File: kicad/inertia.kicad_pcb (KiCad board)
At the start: 2 copper layers, 87.9 x 91.7 mm, 35 parts, among them J10 Conn_01x02, J2 USB_C_Receptacle_USB2.0_16P, J3 Conn_01x02, J4 Conn_01x03, J5 Conn_01x02, J6 Conn_01x03, J7 Conn_01x02, J8 Conn_01x03, J9 Conn_01x02, SW1 SW_Push, SW2 SW_Push, U1 TJA1042T-3, U2 ESP32-S3-WROOM-1, U3 LSM6DSOTR

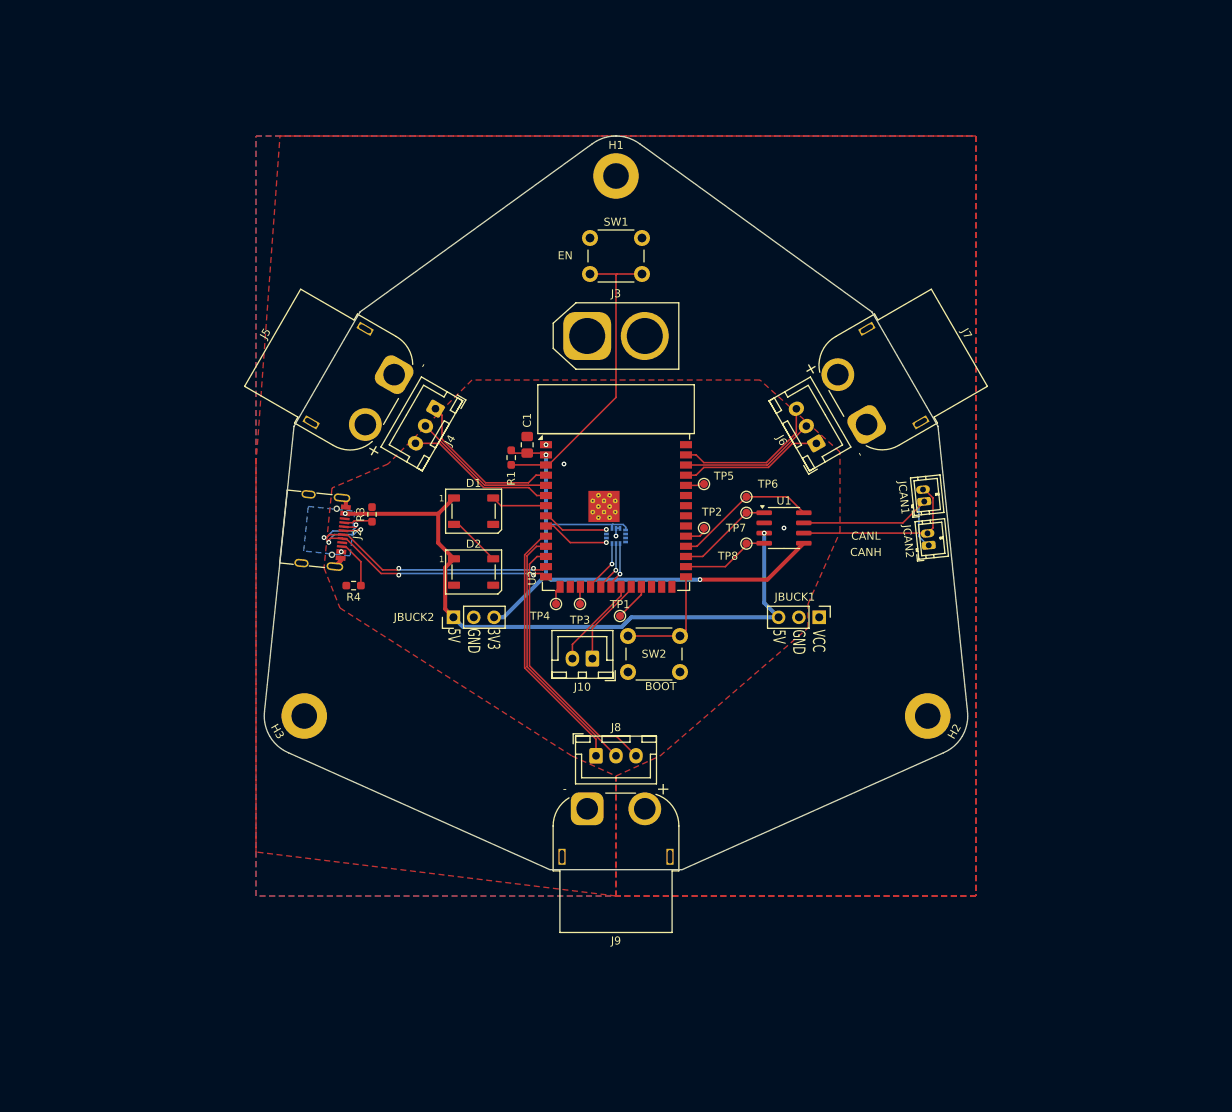
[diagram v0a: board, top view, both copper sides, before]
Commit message: PCB v2
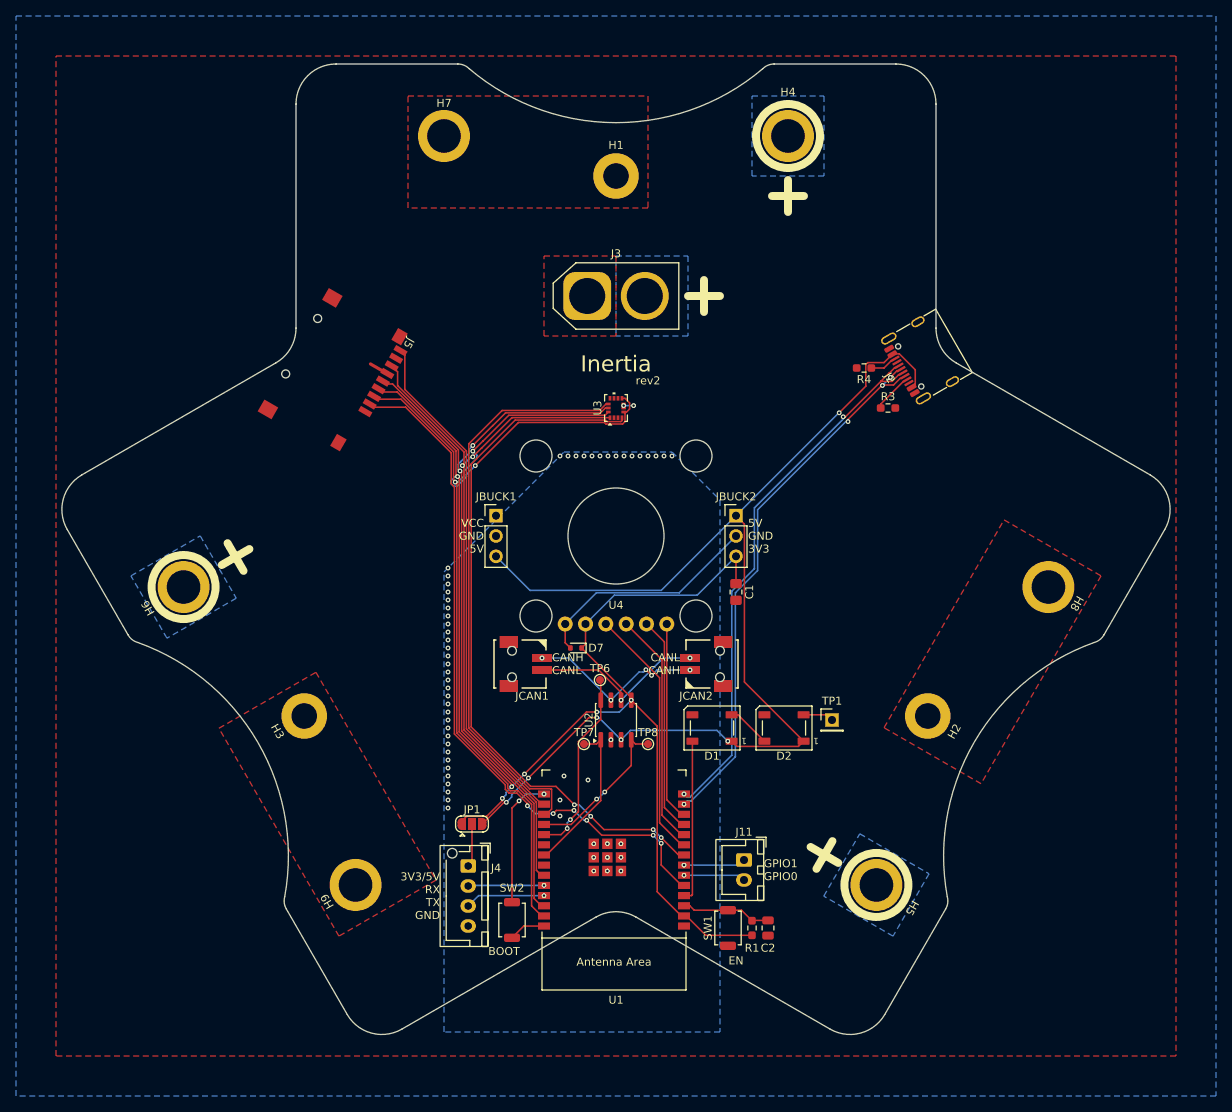
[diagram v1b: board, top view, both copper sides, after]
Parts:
- removed J10: Conn_01x02, Connector_JST:JST_XH_B2B-XH-A_1x02_P2.50mm_Vertical
- removed J6, J8: Conn_01x03, Connector_JST:JST_XH_B3B-XH-A_1x03_P2.50mm_Vertical
- removed J7, J9: Conn_01x02, Connector_AMASS:AMASS_XT60PW-F_1x02_P7.20mm_Horizontal
- removed TP2, TP3, TP4, TP5: TestPoint, TestPoint:TestPoint_Pad_D1.0mm
- added C2: 100nF 6.3V, Capacitor_SMD:C_0805_2012Metric, F.Cu at (19.0, 49.0)
- added D7: ESD5Z3.3T1G, Diode_SMD:D_SOD-523, F.Cu at (-5.00, 14.0)
- added H4: MountingHole_Pad, holes:SMTSOM340, F.Cu at (21.5, -50.0)
- added H5: MountingHole_Pad, holes:SMTSOM340, F.Cu at (32.6, 43.6)
- added H6: MountingHole_Pad, holes:SMTSOM340, F.Cu at (-54.1, 6.38)
- added H7: MountingHole_Pad, holes:SMTSOM340, F.Cu at (-21.5, -50.0)
- added H8: MountingHole_Pad, holes:SMTSOM340, F.Cu at (54.1, 6.38)
- added H9: MountingHole_Pad, holes:SMTSOM340, F.Cu at (-32.6, 43.6)
- added J11: Conn_01x02, Connector_JST:JST_XH_B2B-XH-A_1x02_P2.50mm_Vertical, F.Cu at (16.0, 40.5)
- added JP1: SolderJumper_3_Open, Jumper:SolderJumper-3_P1.3mm_Open_RoundedPad1.0x1.5mm, F.Cu at (-18.0, 36.0)
- added U4: OTOS Robotronik, otos:OTOS_robotronik, F.Cu at (0.00, 0.00)
- C1: value C -> 10uF 6.3V
- J2: value USB_C_Receptacle_USB2.0_16P -> 7010A
- J4: value Conn_01x03 -> Conn_01x04; footprint Connector_JST:JST_XH_B3B-XH-A_1x03_P2.50mm_Vertical -> Connector_JST:JST_XH_B4B-XH-AM_1x04_P2.50mm_Vertical
- J5: value Conn_01x02 -> tf01A; footprint Connector_AMASS:AMASS_XT60PW-F_1x02_P7.20mm_Horizontal -> TF01A:TF-01A
- JCAN1, JCAN2: value Conn_01x02 -> S2B-ZR-SM; footprint Connector_JST:JST_ZH_B2B-ZR_1x02_P1.50mm_Vertical -> jst:S2B-ZR-SMxA
- SW1, SW2: value SW_Push -> TS-1088-AR02016; footprint Button_Switch_THT:SW_PUSH_6mm_H5mm -> Button_Switch_SMD:SW_SPST_TS-1088-xR020
- TP1: footprint TestPoint:TestPoint_Pad_D1.0mm -> Connector_PinHeader_2.54mm:PinHeader_1x01_P2.54mm_Vertical
- U1: value TJA1042T-3 -> ESP32-C5-WROOM-1; footprint Package_SO:SOIC-8_3.9x4.9mm_P1.27mm -> PCM_Espressif:ESP32-C5-WROOM-1
- U2: value ESP32-S3-WROOM-1 -> TJA1042T-3; footprint RF_Module:ESP32-S3-WROOM-1U -> Package_SO:SOIC-8_3.9x4.9mm_P1.27mm
- U3: footprint footprints:LGA-14L_2P5X3X0P86_STM -> LSM6DSO:LGA-14L_2P5X3X0P86_STM; moved to F.Cu
- moved SW1 88.0 mm to (14.0, 49.0), turned to 90 degrees
- moved J2 79.8 mm to (39.0, -22.5), turned to 120 degrees
- moved R4 69.4 mm to (31.0, -21.0)
- moved R1 66.1 mm to (17.0, 49.0), turned to 90 degrees
- moved R3 65.9 mm to (34.0, -16.0), turned to 0 degrees
- moved J4 57.3 mm to (-18.5, 41.2), turned to -90 degrees
- moved JCAN1 54.5 mm to (-12.0, 16.0), turned to -90 degrees
- moved U1 48.8 mm to (0.00, 43.0), turned to 180 degrees
- moved D2 43.4 mm to (21.0, 24.0), turned to 180 degrees
- moved JBUCK1 42.3 mm to (-15.0, -2.54), turned to 0 degrees
- moved D1 40.3 mm to (12.0, 24.0), turned to 180 degrees
- moved JBUCK2 37.5 mm to (15.0, -2.54), turned to 0 degrees
- moved SW2 37.4 mm to (-13.0, 48.0), turned to 90 degrees
- moved TP7 35.3 mm to (-4.00, 26.0)
- moved C1 31.9 mm to (15.0, 7.00), turned to -90 degrees
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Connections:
- C1 pad 1: +3.3V -> +3V3
- D2 pad 2: unconnected-(D2-DOUT-Pad2) -> Net-(D2-DOUT)
- J4 pad 1: ESC0 -> Net-(J4-Pin_1)
- J4 pad 2: TX0 -> /U0RXD
- J4 pad 3: RX0 -> /U0TXD
- J5 pad 1: GND -> unconnected-(J5-DAT2-Pad1)
- J5 pad 2: VCC -> /SD_CS
- JBUCK2 pad 3: +3.3V -> +3V3
- R1 pad 1: +3.3V -> +3V3
- TP1 pad 1: Net-(U2-IO21) -> Net-(D2-DOUT)
- U1 pad 1: /CANTX -> GND
- U1 pad 2: GND -> +3V3
- U1 pad 3: +5V -> /EN
- U1 pad 4: /CANRX -> RGBLED
- U1 pad 5: +3.3V -> /SD_CS
- U1 pad 6: /CAN- -> /GPIO0
- U1 pad 7: /CAN+ -> /GPIO1
- U1 pad 8: /CANSTB -> GY_INT
- U2 pad 1: GND -> /CANTX
- U2 pad 2: +3.3V -> GND
- U2 pad 3: /EN -> +5V
- U2 pad 4: ESC0 -> /CANRX
- U2 pad 5: TX0 -> +3V3
- U2 pad 6: RX0 -> /CAN-
- U2 pad 7: RGBLED -> /CAN+
- U2 pad 8: GY_INT -> /CANSTB
- U3 pad 5: +3.3V -> +3V3
- U3 pad 8: +3.3V -> +3V3
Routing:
- net +3V3: track 0.00 -> 194.1 mm, vias 0 -> 7
- net MOSI: track 6.53 -> 100.6 mm, vias 1 -> 2
- net SCLK: track 6.20 -> 97.6 mm, vias 1 -> 2
- net /SD_CS: track 0.00 -> 87.0 mm, vias 0 -> 6
- net MISO: track 8.40 -> 92.9 mm, vias 1 -> 2
- net GY_INT: track 8.30 -> 87.7 mm, vias 1 -> 4
- net +3.3V: track 73.6 -> 0.00 mm, vias 2 -> 0
- net +5V: track 82.0 -> 151.5 mm, vias 3 -> 6
- net GY_CS: track 5.86 -> 72.3 mm, vias 1 -> 0
- net /SD_DET: track 0.00 -> 64.3 mm
- net RX2: track 33.2 -> 0.00 mm
- net TX2: track 32.5 -> 0.00 mm
- net ESC2: track 32.4 -> 0.00 mm
- net /SDA: track 0.00 -> 31.8 mm
- net /D-: track 36.9 -> 68.5 mm
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- added copper zone on B.Cu, net VCC
- removed copper zone on B.Cu, net +5V
- removed copper zone on F.Cu, net VCC
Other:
- board size 87.9 x 91.7 mm -> 138.5 x 121.3 mm
- board text added: "3V3/5V RX TX GND"
- board text added: "5V GND 3V3"
- board text added: "CANH CANL"
- board text added: "CANL CANH"
- board text added: "GPIO1 GPIO0"
- board text added: "Inertia"
- board text added: "rev2"
- board text removed: "3V3 GND 5V"
- board text removed: "CANH"
- board text removed: "CANL"
